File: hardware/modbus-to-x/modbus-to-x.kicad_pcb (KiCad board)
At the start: 4 copper layers, 53 x 53 mm, 63 parts, among them J1 PWR, J2 UART, J3 Screw_Terminal_3.5mm_2, J4 SSQ-110-X-X-D, SW1 1825910-7, SW2 1825910-7, U1 AMS1117-3.3, U2 ESP32-WROOM-32DM113DH6400PH3Q0, U3 MAX3485, U5 AT24CS64-XHM, U6 AT24CS64-XHM, U7 LMR14020SQDPRTQ1

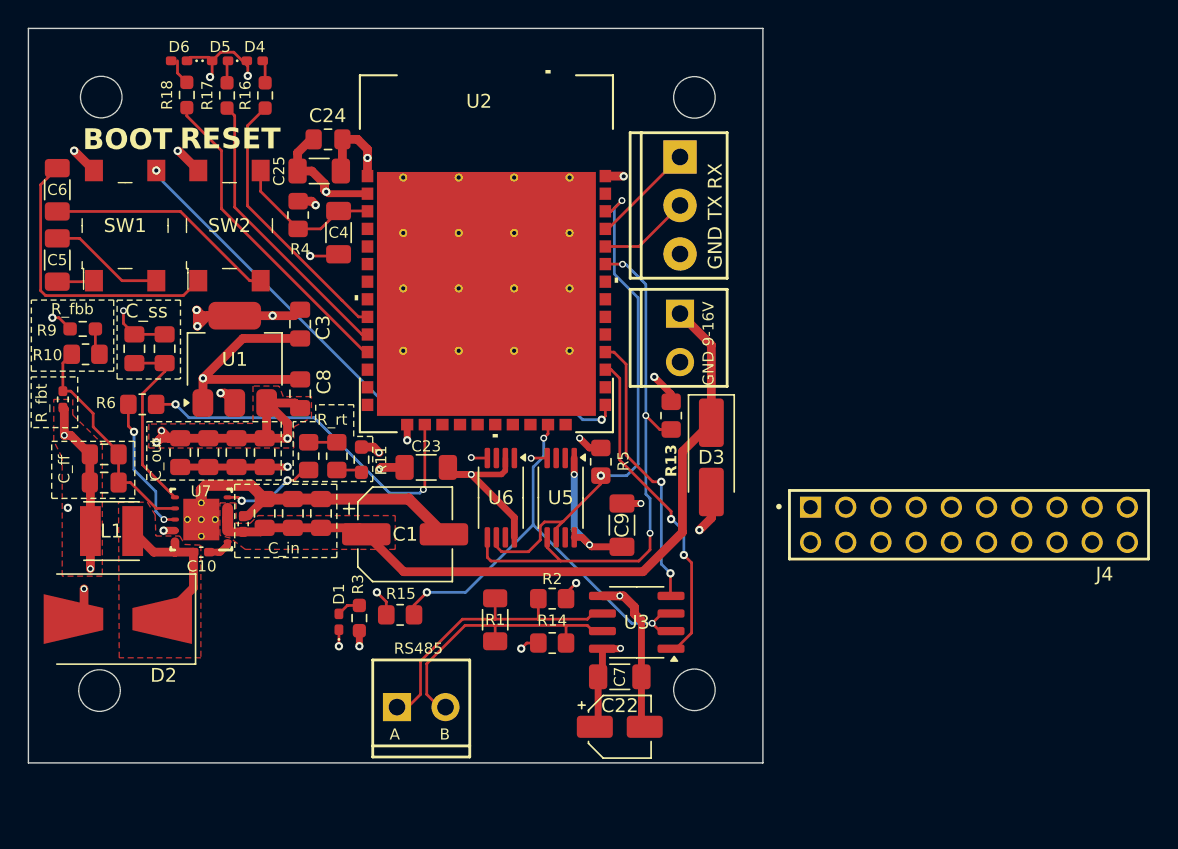
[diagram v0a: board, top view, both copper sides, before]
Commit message: improved edge cuts
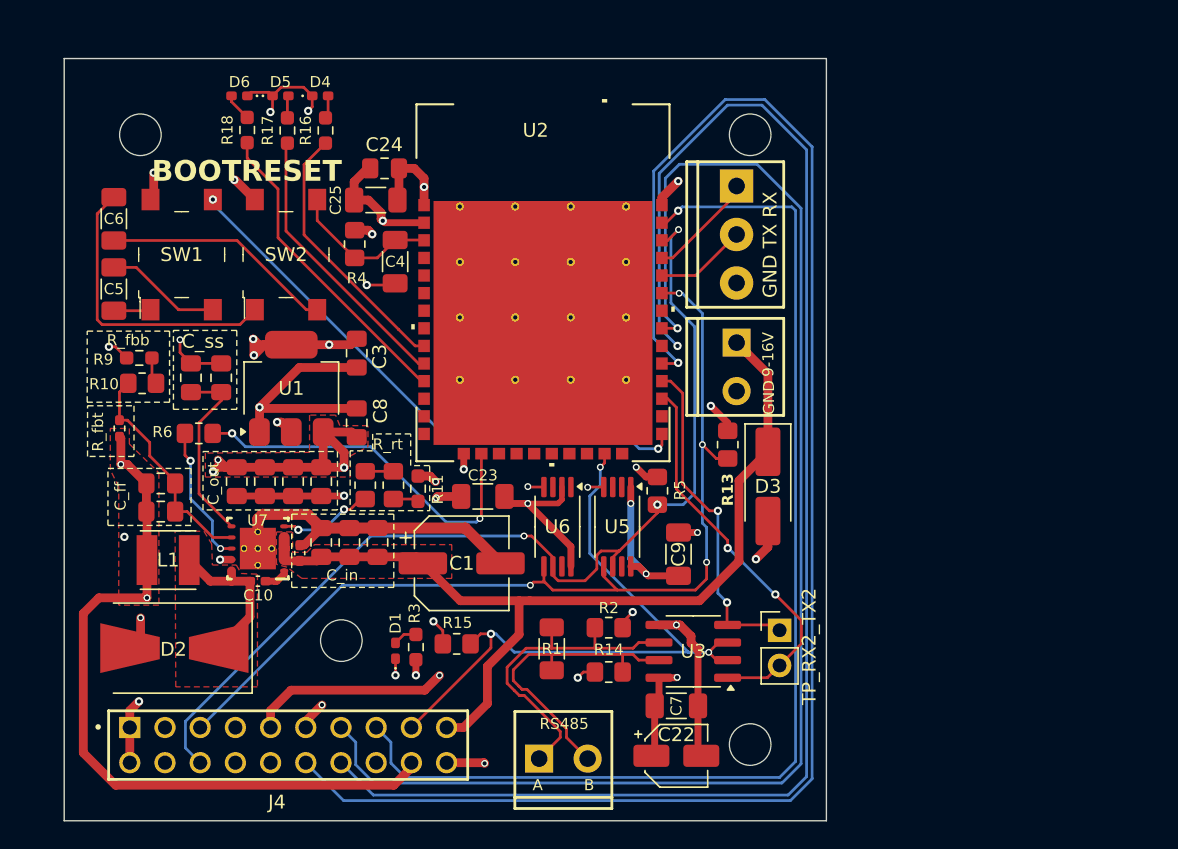
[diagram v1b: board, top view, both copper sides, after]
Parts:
- added TP_RX2_TX2: TestPoint_2Pole, Connector_PinHeader_2.54mm:PinHeader_1x02_P2.54mm_Vertical, F.Cu at (131.6, 121.3)
- moved J4 51.6 mm to (96.2, 129.5)
- moved J3 10.9 mm to (114.3, 130.5)
- moved G*** 6.51 mm to (106.7, 110.6)
- moved D4 5.36 mm to (98.5, 82.7)
- moved D5 5.04 mm to (95.6, 82.7)
- moved R16 5.04 mm to (98.9, 85.2)
- moved R17 5.04 mm to (96.1, 85.2)
- moved R18 5.04 mm to (93.2, 85.2)
- moved D6 5.04 mm to (92.6, 82.7)
- moved C10 4.59 mm to (94.0, 117.7)
- moved C18 4.59 mm to (98.5, 114.9)
- moved C20 4.59 mm to (91.3, 103.0)
- moved C25 4.59 mm to (102.5, 90.2)
- moved C5 4.59 mm to (83.6, 96.6)
- moved D3 4.59 mm to (130.8, 110.9)
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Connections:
- J4 pad 04: /RS485_DE_RE -> unconnected-(J4-Pad04)
- J4 pad 07: /RX_{2} -> unconnected-(J4-Pad07)
- J4 pad 08: /TX_{2} -> unconnected-(J4-Pad08)
- J4 pad 12: unconnected-(J4-Pad12) -> /SPI_CS
- J4 pad 13: /RX_0 -> /SPI_MISO
- J4 pad 14: /TX_0 -> /SPI_CLK
- J4 pad 15: unconnected-(J4-Pad15) -> /SPI_MOSI
- J4 pad 17: unconnected-(J4-Pad17) -> /RS485_DE_RE
- U2 pad 29: unconnected-(U2-IO5-Pad29) -> /SPI_CS
- U2 pad 30: unconnected-(U2-IO18-Pad30) -> /SPI_CLK
- U2 pad 31: unconnected-(U2-IO19-Pad31) -> /SPI_MISO
- U2 pad 37: unconnected-(U2-IO23-Pad37) -> /SPI_MOSI
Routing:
- net /SPI_CS: track 0.00 -> 114.7 mm, vias 0 -> 1
- net /SPI_CLK: track 0.00 -> 107.3 mm, vias 0 -> 1
- net /SPI_MISO: track 0.00 -> 100.3 mm, vias 0 -> 1
- net /SPI_MOSI: track 0.00 -> 83.1 mm, vias 0 -> 1
- net VCC5: track 32.9 -> 73.5 mm
- net /SCL_BUS: track 37.4 -> 74.2 mm, vias 2 -> 3
- net /SDA_BUS: track 40.8 -> 69.9 mm, vias 3 -> 4
- net VDD33: track 61.0 -> 75.5 mm, vias 15 -> 16
- net /RS485_DE_RE: track 34.1 -> 48.1 mm
- net /VBUS_12: track 54.6 -> 66.7 mm
- net GND: track 102.7 -> 113.8 mm, vias 23 -> 26
- net /RX_{2}: track 23.8 -> 28.5 mm
- net /TX_{2}: track 20.3 -> 24.2 mm
- net /RS485-: track 20.4 -> 22.9 mm
- net /RS485+: track 22.0 -> 24.4 mm
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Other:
- board size 53 x 53 mm -> 55 x 55 mm
